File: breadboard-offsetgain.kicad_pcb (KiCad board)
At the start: 2 copper layers, 17.8 x 53.3 mm, 15 parts, among them J1 Conn_02x01, J2 Conn_02x01, J3 Conn_02x01, J4 Conn_02x01, J5 Conn_01x04, J6 Conn_01x04, U1 TL072

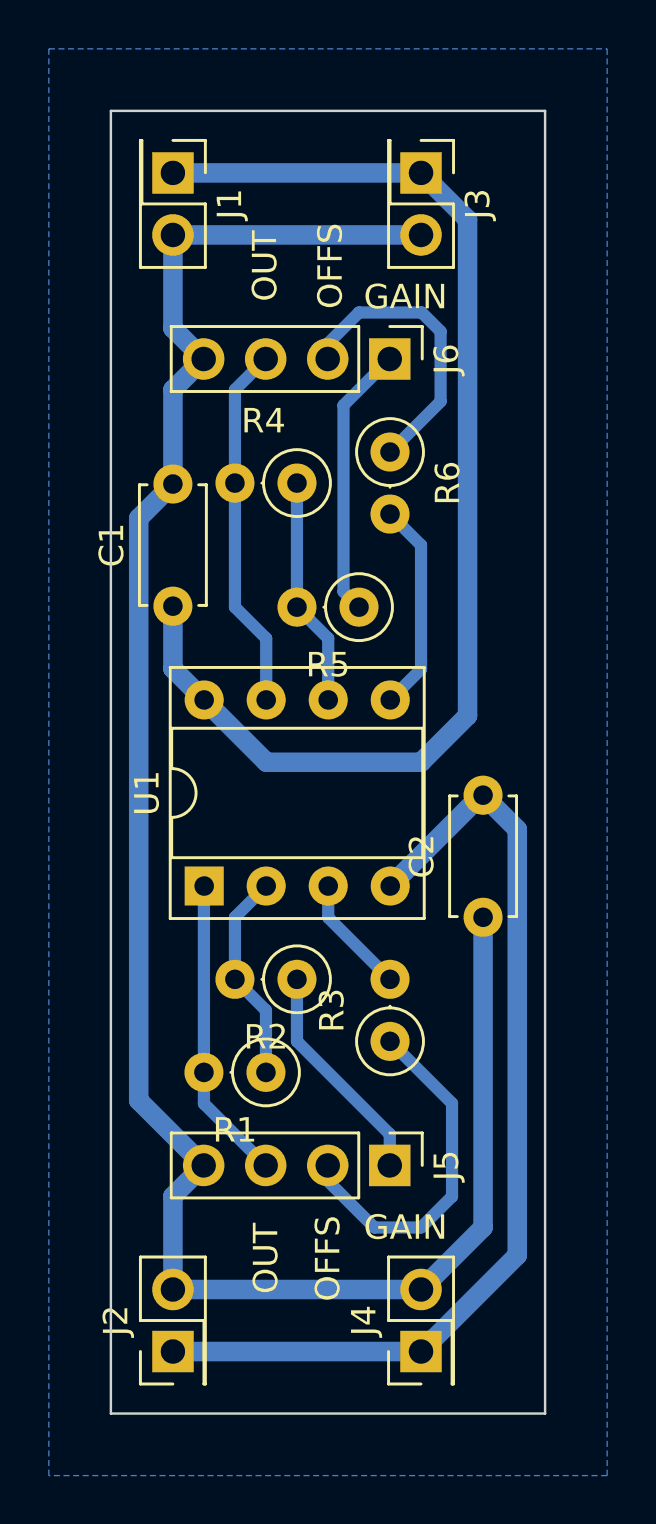
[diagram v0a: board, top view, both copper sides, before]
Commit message: Add image and schematic
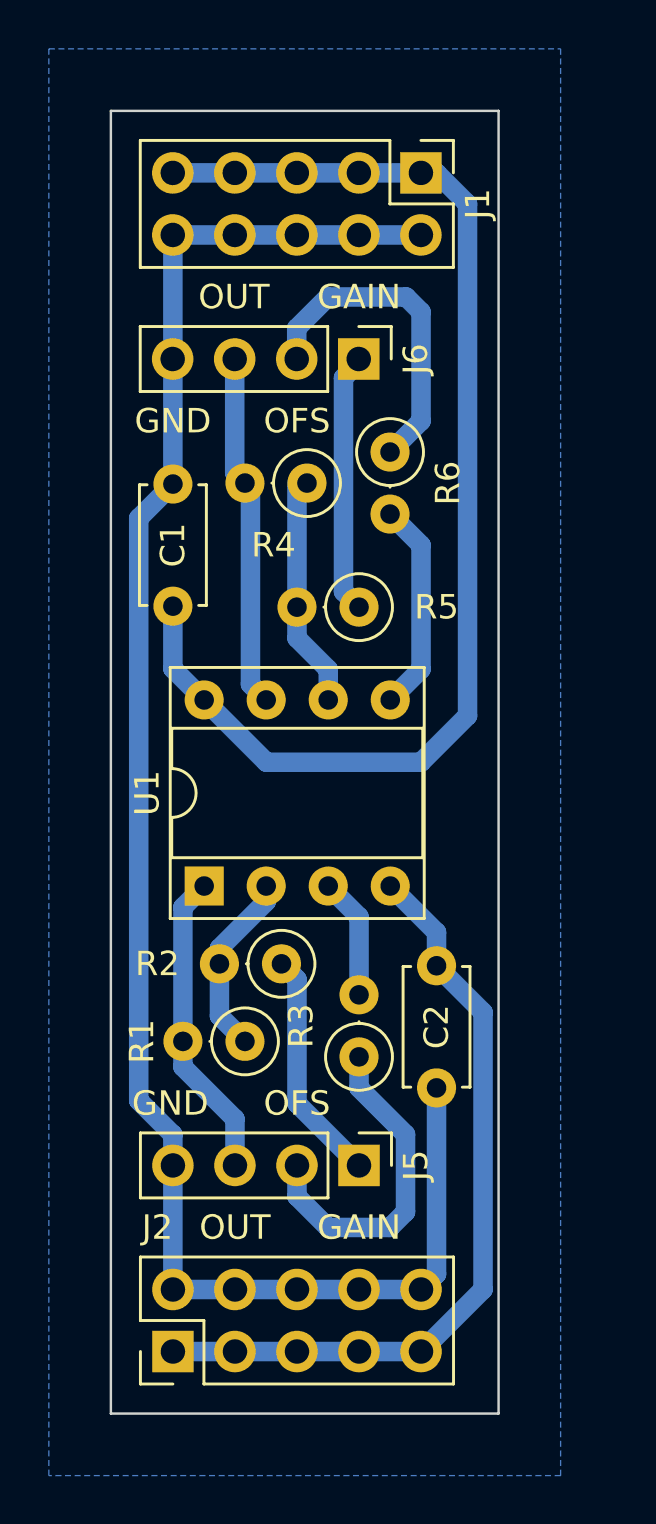
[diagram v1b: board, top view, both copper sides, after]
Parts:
- removed J3, J4: Conn_02x01, Connector_PinHeader_2.54mm:PinHeader_2x01_P2.54mm_Vertical
- J1, J2: value Conn_02x01 -> Conn_02x05; footprint Connector_PinHeader_2.54mm:PinHeader_2x01_P2.54mm_Vertical -> Connector_PinHeader_2.54mm:PinHeader_2x05_P2.54mm_Vertical
- moved J1 10.2 mm to (172.7, 71.1)
- moved C2 7.24 mm to (173.4, 108.6)
- moved R1 1.53 mm to (165.5, 106.7)
- moved R3 1.42 mm to (170.2, 107.3)
- moved J6 1.27 mm to (170.2, 78.7)
- moved J5 1.26 mm to (170.2, 111.8)
- moved R2 0.90 mm to (167.0, 103.5)
- moved R4 0.41 mm to (168.1, 83.8)
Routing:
- net GND: track 83.0 -> 73.2 mm
- net -12V: track 40.5 -> 31.8 mm
- net Net-(J6-Pad2): track 11.9 -> 13.4 mm
- net Net-(R1-Pad1): track 8.69 -> 7.59 mm
- net Net-(J5-Pad2): track 14.4 -> 13.6 mm
- net Net-(J6-Pad1): track 11.2 -> 10.7 mm
- net Net-(J6-Pad3): track 15.0 -> 14.5 mm
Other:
- board size 17.8 x 53.3 mm -> 15.9 x 53.3 mm
- board text added: "GND"
- board text added: "OFS"
- board text removed: "OFFS"
